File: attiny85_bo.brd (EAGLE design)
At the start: 36 x 20 mm, 11 parts, among them IC1 ATTiny85, J1 AVR_SPI_PRG_6NS, Y1 16MHz

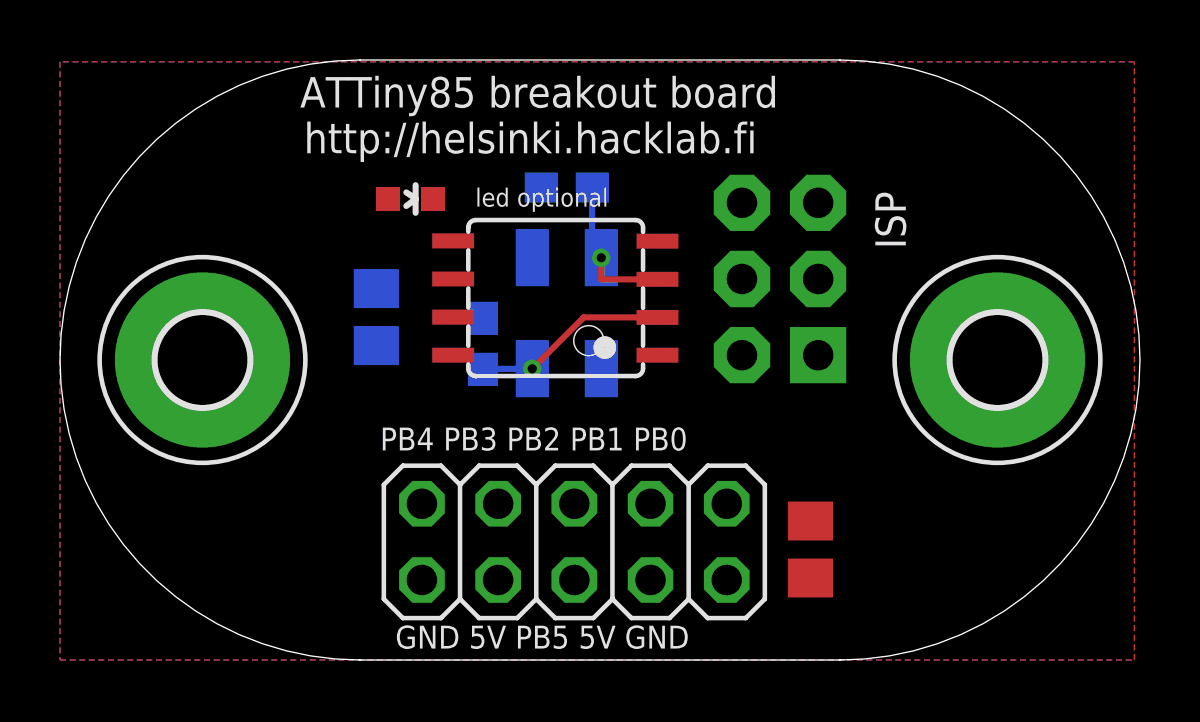
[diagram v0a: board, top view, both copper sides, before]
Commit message: let autorouter take care of the rest
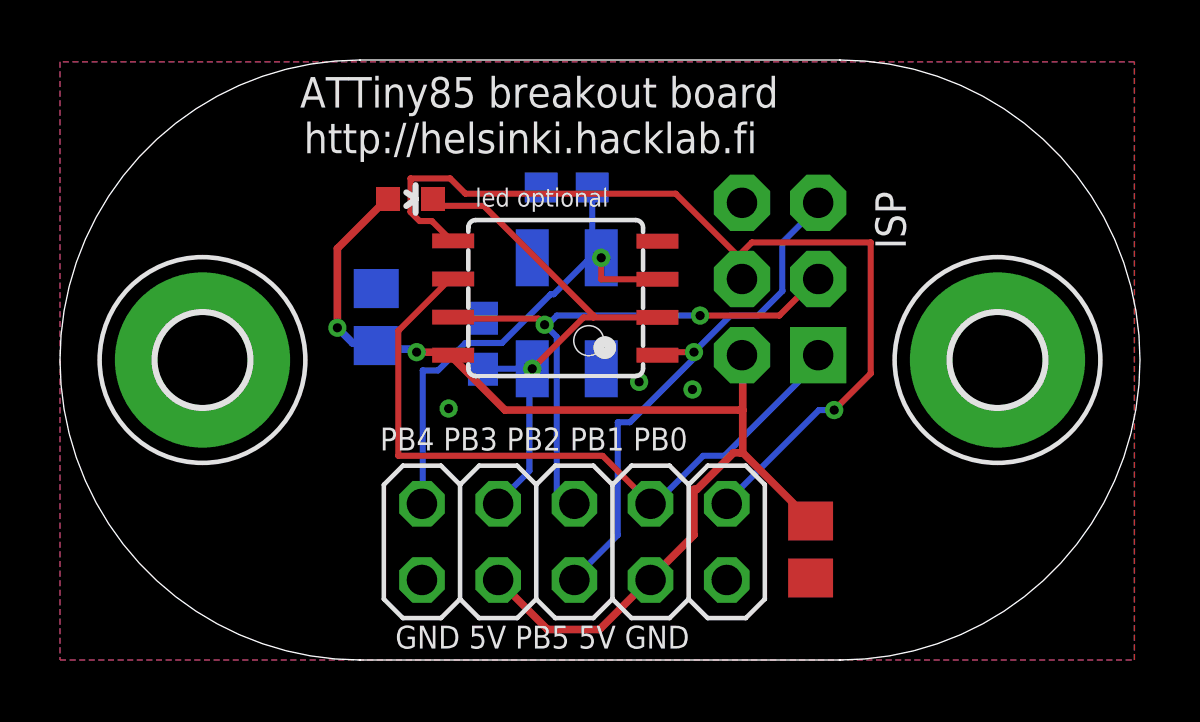
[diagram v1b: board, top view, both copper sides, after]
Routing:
- net +5V: track 0.00 -> 38.4 mm, vias 0 -> 2
- net PB0: track 0.00 -> 32.1 mm, vias 0 -> 1
- net PB1: track 0.00 -> 23.9 mm
- net PB2: track 0.00 -> 19.6 mm, vias 0 -> 2
- net PB5: track 0.00 -> 18.0 mm, vias 0 -> 1
- net PB3: track 6.53 -> 18.5 mm
- net PB4: track 5.23 -> 17.2 mm
